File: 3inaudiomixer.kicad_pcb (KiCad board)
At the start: 2 copper layers, 39 parts, among them J1 AudioJack3, J2 AudioJack3, J3 AudioJack3, U1 LF353D, U2 LF353D, U3 L78L05_SOT89, U4 L79L05_SOT89

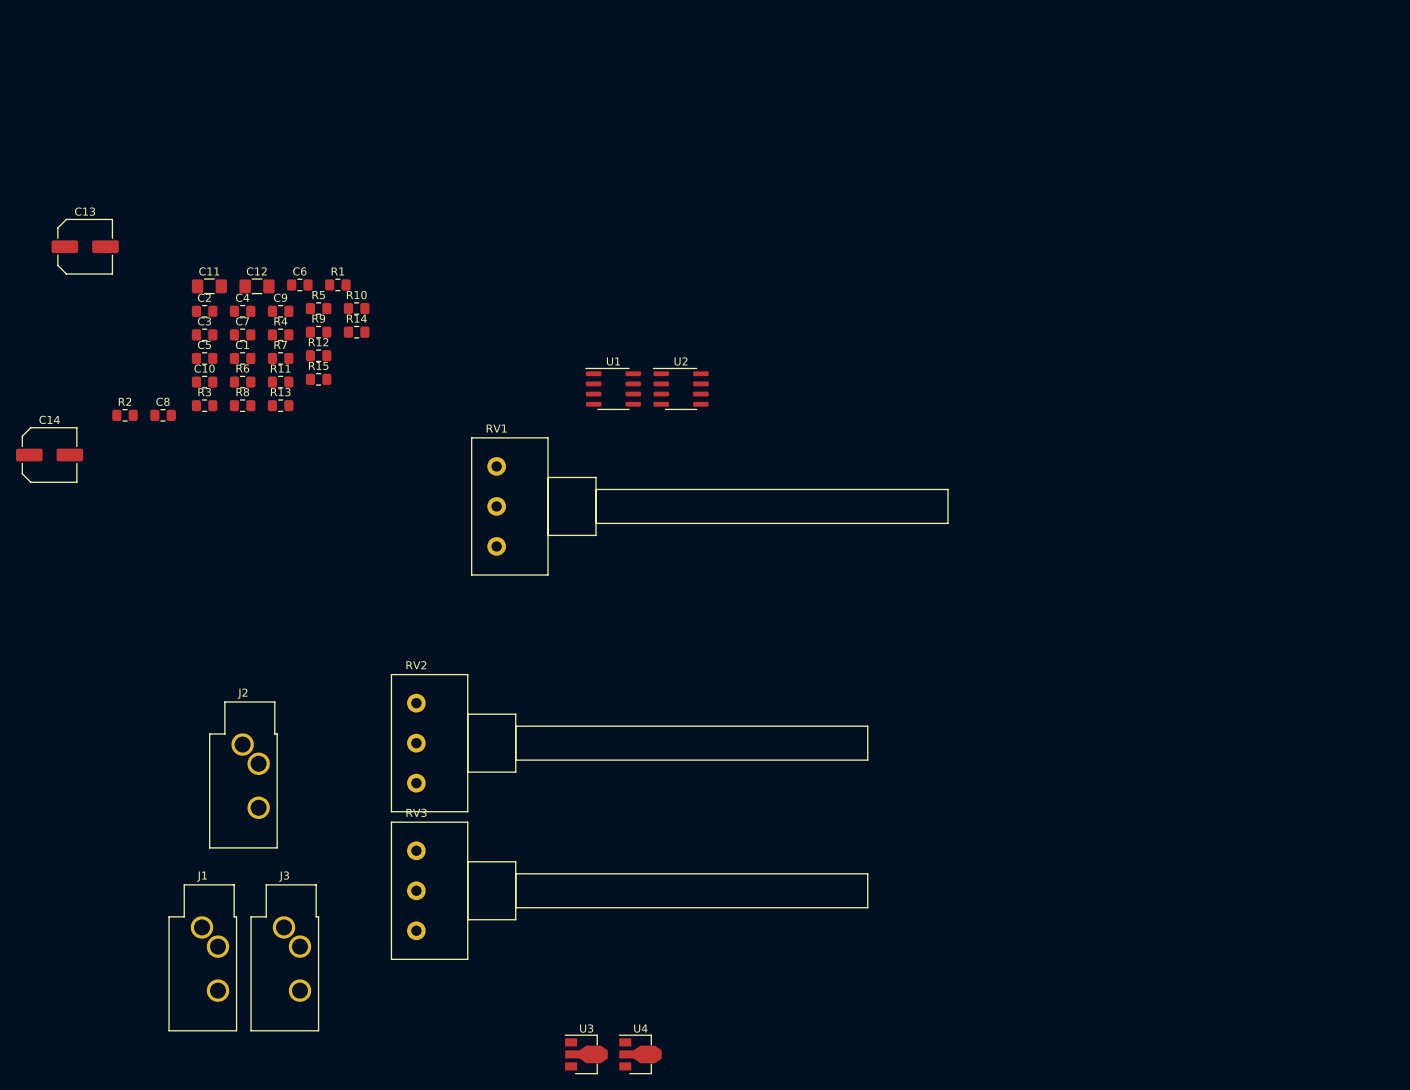
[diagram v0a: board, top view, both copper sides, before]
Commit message: some traces routed
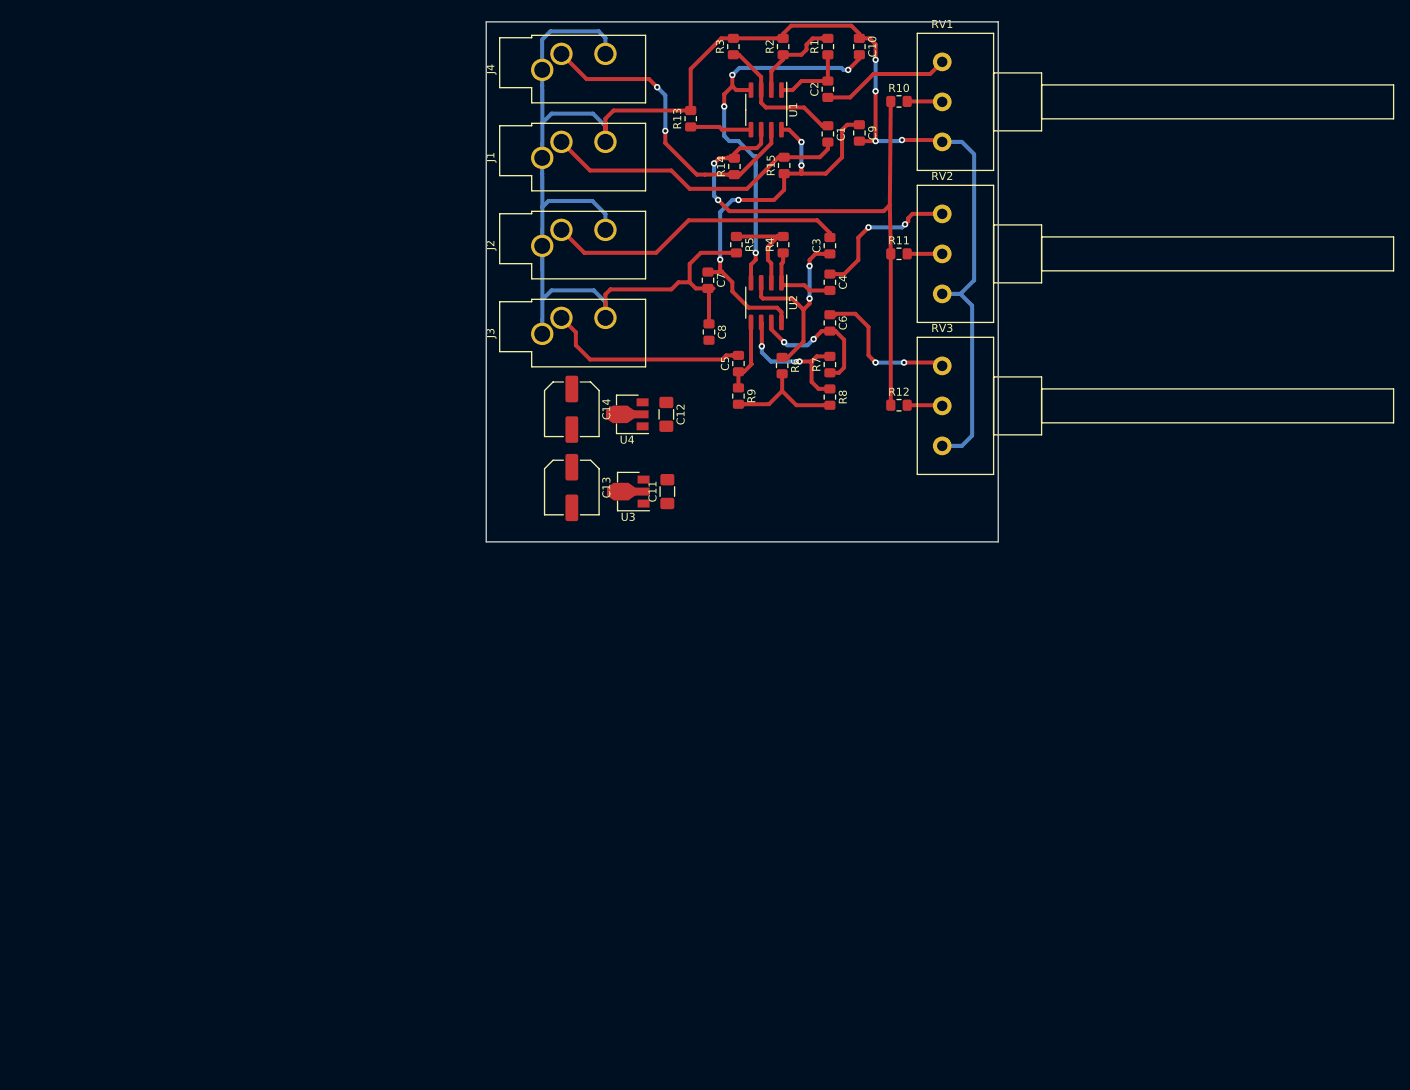
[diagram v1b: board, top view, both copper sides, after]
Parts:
- added J4: AudioJack3, Connector_Audio:Jack_3.5mm_CUI_SJ1-3533NG_Horizontal_CircularHoles, F.Cu at (120.0, 56.0)
- moved J1 105.2 mm to (120.0, 67.0), turned to 90 degrees
- moved R2 94.3 mm to (150.1, 53.1), turned to 90 degrees
- moved C10 92.0 mm to (159.6, 53.1), turned to 270 degrees
- moved RV2 89.8 mm to (170.0, 84.0)
- moved RV3 89.4 mm to (170.0, 103.0)
- moved C2 82.7 mm to (155.7, 58.4), turned to 90 degrees
- moved J3 80.9 mm to (120.0, 89.0), turned to 90 degrees
- moved U4 80.0 mm to (131.1, 99.1), turned to 180 degrees
- moved R3 79.9 mm to (143.9, 53.1), turned to 90 degrees
- moved C3 78.9 mm to (156.0, 78.0), turned to 90 degrees
- moved R11 78.9 mm to (164.6, 79.0)
- moved C1 78.4 mm to (155.7, 64.0), turned to 270 degrees
- moved C9 75.7 mm to (159.6, 63.9), turned to 270 degrees
- moved RV1 75.2 mm to (170.0, 65.0)
- moved C4 73.5 mm to (156.0, 82.5), turned to 270 degrees
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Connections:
- RV3 pad 2: Net-(RV3-Pad2) -> Net-(R12-Pad2)
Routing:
- net Net-(C10-Pad1): track 0.00 -> 247.0 mm, vias 0 -> 4
- net Net-(R10-Pad1): track 0.00 -> 75.0 mm, vias 0 -> 2
- net Net-(C11-Pad1): track 0.00 -> 53.0 mm, vias 0 -> 4
- net Net-(C10-Pad2): track 0.00 -> 49.0 mm, vias 0 -> 4
- net Net-(J4-PadT): track 0.00 -> 39.3 mm, vias 0 -> 2
- net Net-(C1-Pad2): track 0.00 -> 38.7 mm
- net Net-(C3-Pad2): track 0.00 -> 37.7 mm
- net Net-(C5-Pad2): track 0.00 -> 25.4 mm
- net Net-(C3-Pad1): track 0.00 -> 24.6 mm, vias 0 -> 2
- net Net-(C4-Pad1): track 0.00 -> 19.0 mm, vias 0 -> 2
- net Net-(C6-Pad1): track 0.00 -> 18.9 mm, vias 0 -> 2
- net Net-(R7-Pad2): track 0.00 -> 18.2 mm, vias 0 -> 2
- net Net-(C6-Pad2): track 0.00 -> 17.5 mm, vias 0 -> 2
- net Net-(C1-Pad1): track 0.00 -> 17.4 mm
- net Net-(C2-Pad1): track 0.00 -> 16.1 mm
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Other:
- board outline added: 64 x 65 mm
- net class Default: trace_width 0.25 -> 0.5
